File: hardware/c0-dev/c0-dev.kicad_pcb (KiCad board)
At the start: 2 copper layers, 434 parts, among them J101 2913730000, J102 2913710000, J103 2913730000, J104 2913730000, J105 2913710000, J106 2913730000, J107 2913730000, J108 2913710000, J109 2913730000, J110 2913730000, J111 2913730000, J112 2913710000, J113 2913730000, J114 2913730000, J201 RJ45_LED_Shielded, J401 TAG_CONNECT, J402 PinHeader_2.54mm, Q1001 BSS138P, Q1002 BSS138P, Q1003 BSS138P, Q1004 BSS138P, Q1005 BSS138P, Q1006 BSS138P, Q1007 BSS138P, Q1008 BSS138P, Q701 BSS138P, Q702 BSS138P, U1001 B0505S-1WR3, U1002 ISO1540, U1003 TLP175A, U1004 TCA9555PWR, U1005 TPS4H000A-Q1, U1006 TPS4H000A-Q1, U1101 LM5160A, U1102 LM317L, U1201 ER_OLEDM0.91_1x-I2C, U201 LAN8720A, U301 TPS54360DDA, U302 TPS2378, U303 TLP175A, U304 B0505S-1WR3, U305 AMS1117-3.3, U401 TCA9555PWR, U402 W25Q128JVP, U403 TPS3820-33DBV, U404 RP2350A, U501 TMP117xxDRV, U502 B0505S-1WR3, U503 ISO1540, U504 AMS1117-3.3, U505 ADS1015IDGS, U506 ADS1015IDGS, U601 B0505S-1WR3, U602 ISO1540, U603 ADS1015IDGS, U604 ADS1015IDGS, U605 ADS1015IDGS, U606 ADS1015IDGS, U701 B0505S-1WR3, U702 ISO6741, U703 ISO6741, U704 ADS1220xPW, U705 ADS1220xPW, U801 B0505S-1WR3, U802 ISO1044BD, U803 TLP175A, U901 ISO1212, U902 ISO1212, U903 ISO1212, U904 ISO1212, Y401 ABM8-272-T3 (12Mhz)

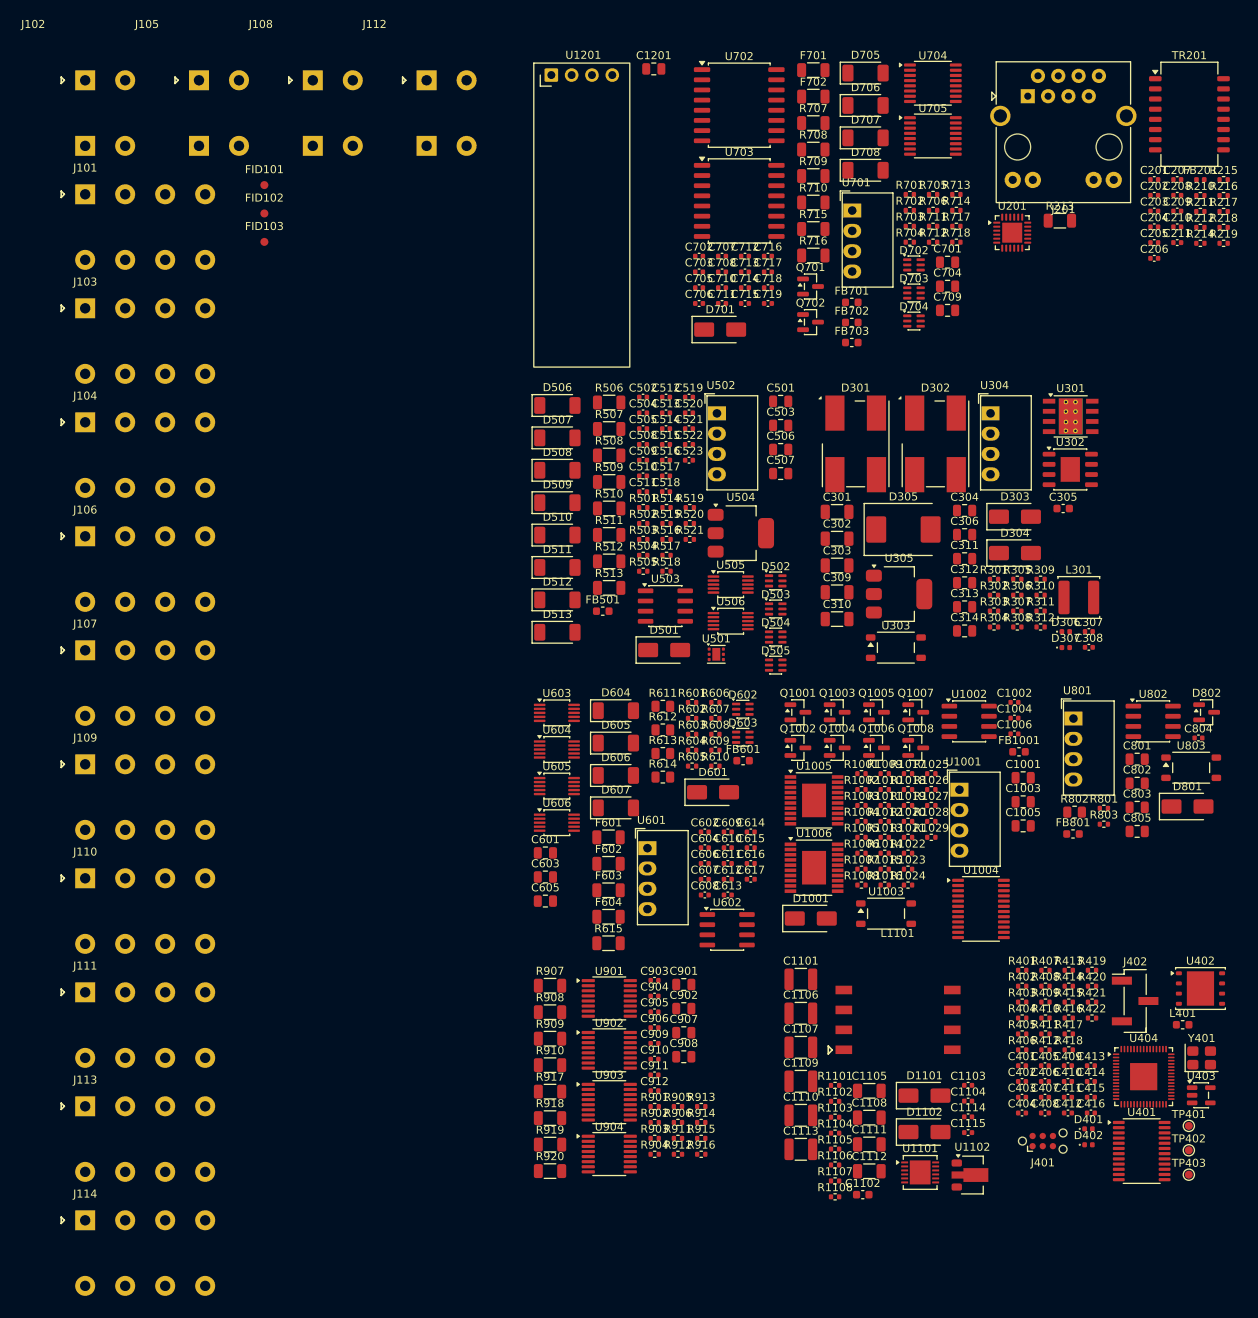
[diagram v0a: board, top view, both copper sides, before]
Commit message: cjc overhaul
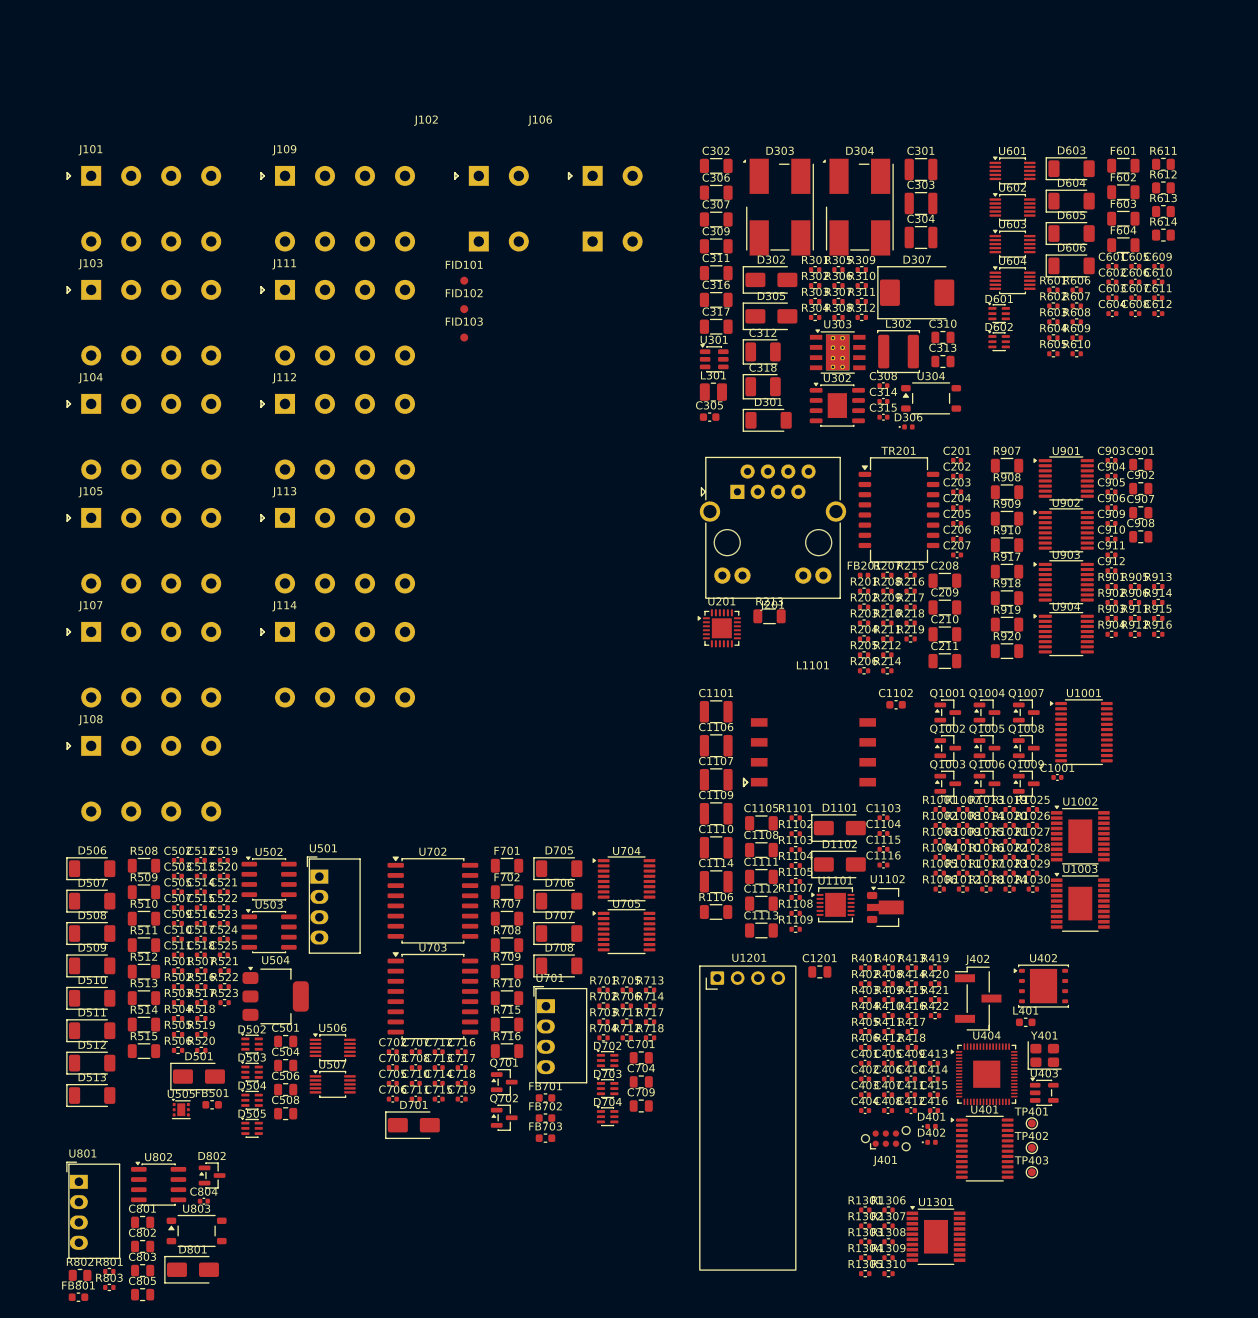
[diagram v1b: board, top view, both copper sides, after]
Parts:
- removed C1002, C1004, C1006, C613, C614, C615, C616, C617: 0.1uF, Capacitor_SMD:C_0402_1005Metric
- removed C1003, C1005: 10uF, Capacitor_SMD:C_0805_2012Metric
- removed D1001: SS14, Diode_SMD:D_SMA
- removed D607: PTVS30VP1UP, Diode_SMD:D_SOD-128
- removed FB1001, FB601: 600Ω@100MHz, Inductor_SMD:L_0603_1608Metric
- removed J110: 2913730000, conduit:2913730000
- removed R615: 0, Resistor_SMD:R_1206_3216Metric
- removed U1004: TCA9555PWR, Package_SO:TSSOP-24_4.4x7.8mm_P0.65mm
- removed U1005, U1006: TPS4H000A-Q1, Package_SO:ETSSOP-20-1EP_4.4x6.5mm_P0.65mm_EP3x4.2mm
- removed U305: AMS1117-3.3, Package_TO_SOT_SMD:SOT-223-3_TabPin2
- removed U605, U606: ADS1015IDGS, Package_SO:TSSOP-10_3x3mm_P0.5mm
- added C1116: 4.7nF, Capacitor_SMD:C_0402_1005Metric, F.Cu at (133.4, 125.0)
- added C315: 3.3nF, Capacitor_SMD:C_0402_1005Metric, F.Cu at (133.4, 69.0)
- added C316: 22uF, Capacitor_SMD:C_1206_3216Metric, F.Cu at (112.5, 54.3)
- added C317: 22uF, Capacitor_SMD:C_1206_3216Metric, F.Cu at (112.5, 57.7)
- added C318: 100uF, Capacitor_Tantalum_SMD:CP_EIA-3528-21_Kemet-B, F.Cu at (118.4, 65.2)
- added C524: 0.1uF, Capacitor_SMD:C_0402_1005Metric, F.Cu at (51.0, 134.2)
- added C525: 0.1uF, Capacitor_SMD:C_0402_1005Metric, F.Cu at (51.0, 136.2)
- added L302: 4.7uH, Inductor_SMD:L_Sunlord_SWPA5040S, F.Cu at (135.3, 60.8)
- added Q1009: BSS138P, Package_TO_SOT_SMD:SOT-23, F.Cu at (151.3, 114.8)
- added R1030: 20k, Resistor_SMD:R_0402_1005Metric, F.Cu at (152.1, 128.0)
- added R1109: 51k, Resistor_SMD:R_0402_1005Metric, F.Cu at (122.5, 133.0)
- added R1301: 1k, Resistor_SMD:R_0402_1005Metric, F.Cu at (131.2, 168.1)
- added R1302: 1k, Resistor_SMD:R_0402_1005Metric, F.Cu at (131.2, 170.1)
- added R1303: 1k, Resistor_SMD:R_0402_1005Metric, F.Cu at (131.2, 172.1)
- added R1304: 1k, Resistor_SMD:R_0402_1005Metric, F.Cu at (131.2, 174.1)
- added R1305: 2.4k, Resistor_SMD:R_0402_1005Metric, F.Cu at (131.2, 176.0)
- added R1306: 1k, Resistor_SMD:R_0402_1005Metric, F.Cu at (134.1, 168.1)
- added R1307: 1k, Resistor_SMD:R_0402_1005Metric, F.Cu at (134.1, 170.1)
- added R1308: 4.7k, Resistor_SMD:R_0402_1005Metric, F.Cu at (134.1, 172.1)
- added R1309: 20k, Resistor_SMD:R_0402_1005Metric, F.Cu at (134.1, 174.1)
- added R1310: 20k, Resistor_SMD:R_0402_1005Metric, F.Cu at (134.1, 176.0)
- added R201: 10k, Resistor_SMD:R_0402_1005Metric, F.Cu at (131.0, 90.7)
- added R202: 1k, Resistor_SMD:R_0402_1005Metric, F.Cu at (131.0, 92.7)
- added R203: 10R, Resistor_SMD:R_0402_1005Metric, F.Cu at (131.0, 94.7)
- added R204: 10R, Resistor_SMD:R_0402_1005Metric, F.Cu at (131.0, 96.7)
- added R205: 10R, Resistor_SMD:R_0402_1005Metric, F.Cu at (131.0, 98.7)
- added R206: 10R, Resistor_SMD:R_0402_1005Metric, F.Cu at (131.0, 100.7)
- added R207: 33R, Resistor_SMD:R_0402_1005Metric, F.Cu at (133.9, 88.7)
- added R208: 12.1k, Resistor_SMD:R_0402_1005Metric, F.Cu at (133.9, 90.7)
- added R209: 49.9R, Resistor_SMD:R_0402_1005Metric, F.Cu at (133.9, 92.7)
- added R522: 1M, Resistor_SMD:R_0402_1005Metric, F.Cu at (51.1, 140.2)
- added R523: 1M, Resistor_SMD:R_0402_1005Metric, F.Cu at (51.1, 142.2)
- added U1301: TPS4H000A-Q1, Package_SO:ETSSOP-20-1EP_4.4x6.5mm_P0.65mm_EP3x4.2mm, F.Cu at (140.0, 171.4)
- added U507: ADS1015IDGS, Package_SO:TSSOP-10_3x3mm_P0.5mm, F.Cu at (64.6, 152.4)
- C1001, C503, C507, C605: value 10uF -> 0.1uF; footprint Capacitor_SMD:C_0805_2012Metric -> Capacitor_SMD:C_0402_1005Metric
- C1113: value 10uF -> 1nF; footprint Capacitor_SMD:C_1210_3225Metric -> Capacitor_SMD:C_1206_3216Metric
- C1114: value 10nF -> 10uF; footprint Capacitor_SMD:C_0402_1005Metric -> Capacitor_SMD:C_1210_3225Metric
- C1115: value 4.7nF -> 10nF
- C208, C209, C210, C211: value 22nF -> 1nF; footprint Capacitor_SMD:C_0402_1005Metric -> Capacitor_SMD:C_1206_3216Metric
- C301, C303: value 1uF -> 10uF; footprint Capacitor_SMD:C_1206_3216Metric -> Capacitor_SMD:C_1210_3225Metric
- C302: value 1uF -> 22uF
- C304: value 0.1uF -> 10uF; footprint Capacitor_SMD:C_0805_2012Metric -> Capacitor_SMD:C_1210_3225Metric
- C306: value 0.1uF -> 1uF; footprint Capacitor_SMD:C_0805_2012Metric -> Capacitor_SMD:C_1206_3216Metric
- C307: value 270pF -> 1uF; footprint Capacitor_SMD:C_0402_1005Metric -> Capacitor_SMD:C_1206_3216Metric
- C308: value 3.3nF -> 0.1uF
- C309: value 22uF -> 1uF
- C310: value 22uF -> 0.1uF; footprint Capacitor_SMD:C_1206_3216Metric -> Capacitor_SMD:C_0805_2012Metric
- C311: value 10uF -> 22uF; footprint Capacitor_SMD:C_0805_2012Metric -> Capacitor_SMD:C_1206_3216Metric
- C312: value 10uF -> 100uF; footprint Capacitor_SMD:C_0805_2012Metric -> Capacitor_Tantalum_SMD:CP_EIA-3528-21_Kemet-B
- C313: value 10uF -> 0.1uF
- C314: value 10uF -> 270pF; footprint Capacitor_SMD:C_0805_2012Metric -> Capacitor_SMD:C_0402_1005Metric
- C504: value 0.1uF -> 10uF; footprint Capacitor_SMD:C_0402_1005Metric -> Capacitor_SMD:C_0805_2012Metric
- C508: value 1uF -> 10uF; footprint Capacitor_SMD:C_0402_1005Metric -> Capacitor_SMD:C_0805_2012Metric
- C510, C602, C604: value 0.1uF -> 1uF
- C601, C603: value 10uF -> 1uF; footprint Capacitor_SMD:C_0805_2012Metric -> Capacitor_SMD:C_0402_1005Metric
- C606, C607, C608, C609: value 1uF -> 0.1uF
- D301: value CD-DF406SL -> PTVS30VP1UP; footprint Diode_SMD:Diode_Bridge_Bourns_CD-DF4xxS -> Diode_SMD:D_SOD-128
- D302: value CD-DF406SL -> SS14; footprint Diode_SMD:Diode_Bridge_Bourns_CD-DF4xxS -> Diode_SMD:D_SMA
- D303: value SMAJ58A -> CD-DF406SL; footprint Diode_SMD:D_SMA -> Diode_SMD:Diode_Bridge_Bourns_CD-DF4xxS
- D304: value SS14 -> CD-DF406SL; footprint Diode_SMD:D_SMA -> Diode_SMD:Diode_Bridge_Bourns_CD-DF4xxS
- D305: value B560C -> SMAJ58A; footprint Diode_SMD:D_SMC -> Diode_SMD:D_SMA
- D307: value green -> B560C; footprint LED_SMD:LED_0402_1005Metric -> Diode_SMD:D_SMC
- D601: value SS14 -> BAV199DW; footprint Diode_SMD:D_SMA -> Package_TO_SOT_SMD:SOT-363_SC-70-6
- D603: value BAV199DW -> PTVS30VP1UP; footprint Package_TO_SOT_SMD:SOT-363_SC-70-6 -> Diode_SMD:D_SOD-128
- J105, J108, J112: value 2913710000 -> 2913730000; footprint conduit:2913710000 -> conduit:2913730000
- J106: value 2913730000 -> 2913710000; footprint conduit:2913730000 -> conduit:2913710000
- L301: value 4.7uH -> 2.2uH; footprint Inductor_SMD:L_Sunlord_SWPA5040S -> Inductor_SMD:L_1008_2520Metric
- R1001, R1002, R1009, R1012: value 1k -> 4.7k
- R1007: value 10k -> 1k
- R1008: value 4.7k -> 10k
- R1011: value 4.7k -> 1k
- R1022: value 20k -> 1k
- R1106: value 27k -> 2M; footprint Resistor_SMD:R_0402_1005Metric -> Resistor_SMD:R_1206_3216Metric
- R1107: value 2.4k -> 27k
- R1108: value 51k -> 2.4k
- R301: value 68.1k -> 1k
- R302: value 0 -> 25k
- R303: value 25k -> 63.4R
- R304: value 63.4R -> 68.1k
- R305: value 6.34k -> 1k
- R306: value 60.4k -> 1k
- R307: value 11.5k -> 10k
- R309: value 10k -> 6.34k
- R310: value 1k -> 60.4k
- R311: value 1k -> 11.5k
- R506, R507: value 2k -> 1k; footprint Resistor_SMD:R_1206_3216Metric -> Resistor_SMD:R_0402_1005Metric
- R514, R515: value 1M -> 2k; footprint Resistor_SMD:R_0402_1005Metric -> Resistor_SMD:R_1206_3216Metric
- R611, R612, R613, R614: value 160 -> 82
- U1001: value B0505S-1WR3 -> TCA9555PWR; footprint Converter_DCDC:Converter_DCDC_Murata_MEE1SxxxxSC_THT -> Package_SO:TSSOP-24_4.4x7.8mm_P0.65mm
- U1002: value ISO1540 -> TPS4H000A-Q1; footprint Package_SO:SOIC-8_3.9x4.9mm_P1.27mm -> Package_SO:ETSSOP-20-1EP_4.4x6.5mm_P0.65mm_EP3x4.2mm
- U1003: value TLP175A -> TPS4H000A-Q1; footprint Package_SO:Toshiba_SOIC-4-6_4.4x3.6mm_P1.27mm -> Package_SO:ETSSOP-20-1EP_4.4x6.5mm_P0.65mm_EP3x4.2mm
- U301: value TPS54360DDA -> AP63203WU; footprint Package_SO:TI_SO-PowerPAD-8_ThermalVias -> Package_TO_SOT_SMD:TSOT-23-6
- U303: value TLP175A -> TPS54360DDA; footprint Package_SO:Toshiba_SOIC-4-6_4.4x3.6mm_P1.27mm -> Package_SO:TI_SO-PowerPAD-8_ThermalVias
- U304: value B0505S-1WR3 -> TLP175A; footprint Converter_DCDC:Converter_DCDC_Murata_MEE1SxxxxSC_THT -> Package_SO:Toshiba_SOIC-4-6_4.4x3.6mm_P1.27mm
- U501: value TMP117xxDRV -> B0505S-1WR3; footprint Package_SON:WSON-6-1EP_2x2mm_P0.65mm_EP1x1.6mm -> Converter_DCDC:Converter_DCDC_Murata_MEE1SxxxxSC_THT
- U502: value B0505S-1WR3 -> ISO1540; footprint Converter_DCDC:Converter_DCDC_Murata_MEE1SxxxxSC_THT -> Package_SO:SOIC-8_3.9x4.9mm_P1.27mm
- U505: value ADS1015IDGS -> TMP117xxDRV; footprint Package_SO:TSSOP-10_3x3mm_P0.5mm -> Package_SON:WSON-6-1EP_2x2mm_P0.65mm_EP1x1.6mm
- U601: value B0505S-1WR3 -> ADS1015IDGS; footprint Converter_DCDC:Converter_DCDC_Murata_MEE1SxxxxSC_THT -> Package_SO:TSSOP-10_3x3mm_P0.5mm
- U602: value ISO1540 -> ADS1015IDGS; footprint Package_SO:SOIC-8_3.9x4.9mm_P1.27mm -> Package_SO:TSSOP-10_3x3mm_P0.5mm
- moved C802 137.1 mm to (40.8, 172.6)
- moved C804 137.1 mm to (48.5, 167.0)
- moved D801 137.1 mm to (47.1, 175.6)
- moved D802 137.1 mm to (49.5, 163.8)
- moved FB801 137.1 mm to (32.8, 179.0)
- moved R801 137.1 mm to (36.7, 175.8)
- moved R802 137.1 mm to (33.0, 176.3)
- moved U803 137.1 mm to (47.6, 170.7)
- moved C801 137.1 mm to (40.8, 169.6)
- moved C803 137.1 mm to (40.8, 175.7)
- moved C805 137.1 mm to (40.8, 178.7)
- moved R803 137.1 mm to (36.7, 177.8)
- moved U801 137.1 mm to (32.9, 164.6)
- moved U802 137.1 mm to (42.8, 164.9)
- moved U1201 114.8 mm to (112.7, 139.1)
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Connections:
- net /frontend_temp/+5V renamed /frontend_temp/+5V_ISO
- C1001 pad 1: +5V_ISO -> +3.3V
- C1001 pad 2: GND_ISO -> GND
- C1101 pad 2: GND_ISO -> /Power/GND_ISO
- C1102 pad 2: GND_ISO -> /Power/GND_ISO
- C1103 pad 2: GND_ISO -> /Power/GND_ISO
- C1105 pad 2: GND_ISO -> /Power/GND_ISO
- C1106 pad 1: /Power/FlyBuck/+24V -> +24V
- C1106 pad 2: /Power/FlyBuck/GND -> GND
- C1107 pad 1: /Power/FlyBuck/+24V -> +24V
- C1107 pad 2: /Power/FlyBuck/GND -> GND
- C1108 pad 1: /Power/FlyBuck/+24V -> +24V
- C1108 pad 2: /Power/FlyBuck/GND -> GND
- C1109 pad 1: /Power/FlyBuck/+24V -> +24V
- C1109 pad 2: /Power/FlyBuck/GND -> GND
- C1110 pad 1: /Power/FlyBuck/+24V -> +24V
- C1110 pad 2: /Power/FlyBuck/GND -> GND
- C1111 pad 1: /Power/FlyBuck/+24V -> +24V
- C1111 pad 2: /Power/FlyBuck/GND -> GND
- C1112 pad 1: /Power/FlyBuck/+24V -> +24V
- C1112 pad 2: GND_ISO -> /Power/GND_ISO
- C1113 pad 1: /Power/FlyBuck/+24V -> GND
- C1113 pad 2: GND_ISO -> Earth
- C1114 pad 1: /Power/FlyBuck/A -> +24V
- C1114 pad 2: /Power/FlyBuck/FB -> /Power/GND_ISO
- C1115 pad 2: GND_ISO -> /Power/FlyBuck/FB
- C301 pad 1: +POE -> +24V
- C301 pad 2: GND_ISO -> GND
- C302 pad 1: +POE -> +5V
- C302 pad 2: GND_ISO -> GND
- C303 pad 1: +POE -> +24V
- C303 pad 2: GND_ISO -> GND
- C304 pad 1: +POE -> +24V
- C304 pad 2: GND_ISO -> GND
- C306 pad 1: Net-(U301-BOOT) -> +24V
- C306 pad 2: Net-(D305-K) -> GND
- C307 pad 1: Net-(U301-COMP) -> +24V
- C307 pad 2: GND_ISO -> GND
- C308 pad 1: Net-(C308-Pad1) -> Net-(U301-SW)
- C308 pad 2: GND_ISO -> Net-(U301-BST)
- C309 pad 1: +5V_ISO -> +24V
- C309 pad 2: GND_ISO -> GND
- C310 pad 1: +5V_ISO -> +24V
- C310 pad 2: GND_ISO -> GND
- C311 pad 1: +5V_ISO -> GND
- C311 pad 2: GND_ISO -> +3.3V
- C312 pad 1: +5V -> +3.3V
- C313 pad 1: +5V -> Net-(U303-BOOT)
- C313 pad 2: GND -> Net-(D307-K)
- C314 pad 1: +3.3V -> Net-(U303-COMP)
- C501 pad 1: +5V_ISO -> +5V
- C501 pad 2: GND_ISO -> GND
- C503 pad 1: unconnected-(C503-Pad1) -> +3.3V
- C504 pad 1: +3.3V -> unconnected-(C504-Pad1)
- C512 pad 1: Net-(D502B-K1A2) -> +3.3V
- C513 pad 1: Net-(D502B-K1A2) -> +3.3V
- C513 pad 2: Net-(D502A-K3A4) -> GND
- C514 pad 1: Net-(D502A-K3A4) -> Net-(D502B-K1A2)
- C515 pad 1: Net-(D503B-K1A2) -> Net-(D502B-K1A2)
- C515 pad 2: GND -> Net-(D502A-K3A4)
- C516 pad 1: Net-(D503B-K1A2) -> Net-(D502A-K3A4)
- C516 pad 2: Net-(D503A-K3A4) -> GND
- C517 pad 1: Net-(D503A-K3A4) -> Net-(D503B-K1A2)
- C518 pad 1: Net-(D504B-K1A2) -> Net-(D503B-K1A2)
- C518 pad 2: GND -> Net-(D503A-K3A4)
- C519 pad 1: Net-(D504B-K1A2) -> Net-(D503A-K3A4)
- C519 pad 2: Net-(D504A-K3A4) -> GND
- C520 pad 1: Net-(D504A-K3A4) -> Net-(D504B-K1A2)
- C521 pad 1: Net-(D505B-K1A2) -> Net-(D504B-K1A2)
- C521 pad 2: GND -> Net-(D504A-K3A4)
- C522 pad 1: Net-(D505B-K1A2) -> Net-(D504A-K3A4)
- C522 pad 2: Net-(D505A-K3A4) -> GND
- C523 pad 1: Net-(D505A-K3A4) -> Net-(D505B-K1A2)
- C601 pad 1: +5V_ISO -> +3.3V
- C601 pad 2: GND_ISO -> GND
- C603 pad 1: Net-(U601-+Vout) -> +3.3V
- C604 pad 1: /frontend_420/+5V -> +3.3V
- C605 pad 1: /frontend_420/+5V -> +3.3V
- C606 pad 1: /frontend_420/+5V -> +3.3V
- C607 pad 1: /frontend_420/+5V -> +3.3V
- C608 pad 1: /frontend_420/+5V -> +3.3V
- C609 pad 1: /frontend_420/+5V -> GND
- C609 pad 2: GND -> Net-(U601-AIN0)
- C610 pad 1: /frontend_420/+5V -> GND
- C610 pad 2: GND -> Net-(U602-AIN0)
- C611 pad 1: /frontend_420/+5V -> GND
- C611 pad 2: GND -> Net-(U603-AIN0)
- C612 pad 1: /frontend_420/+5V -> GND
- C612 pad 2: GND -> Net-(U604-AIN0)
- C903 pad 2: /Digital Input/GND_IN -> GND
- C904 pad 2: /Digital Input/GND_IN -> GND
- C905 pad 2: /Digital Input/GND_IN -> GND
- C906 pad 2: /Digital Input/GND_IN -> GND
- C909 pad 2: /Digital Input/GND_IN -> GND
- C910 pad 2: /Digital Input/GND_IN -> GND
- C911 pad 2: /Digital Input/GND_IN -> GND
- C912 pad 2: /Digital Input/GND_IN -> GND
- D1101 pad 1: /Power/FlyBuck/+24V -> +24V
- D1102 pad 1: /Power/FlyBuck/+24V -> +24V
- D301 pad 1: +POE -> GND
- D301 pad 2: /Ethernet/POE+12 -> /Power/V+
- D302 pad 1: +POE -> +24V
- D302 pad 2: /Ethernet/POE+45 -> /Power/V+
- D303 pad 2: -POE -> /Ethernet/POE+12
- D304 pad 2: /Power/V+ -> /Ethernet/POE+45
- D305 pad 1: Net-(D305-K) -> +POE
- D305 pad 2: GND_ISO -> -POE
- D306 pad 1: GND_ISO -> GND
- D307 pad 1: GND -> Net-(D307-K)
- D307 pad 2: Net-(D307-A) -> GND
- D601 pad 1: /frontend_420/+5V -> GND
- D601 pad 2: Net-(D601-A) -> +3.3V
- D602 pad 2: /frontend_420/+5V -> +3.3V
- D602 pad 5: /frontend_420/+5V -> +3.3V
- D603 pad 1: GND -> /frontend_420/4200
- D603 pad 2: /frontend_420/+5V -> GND
- D604 pad 1: /frontend_420/4200 -> /frontend_420/4201
- D605 pad 1: /frontend_420/4201 -> /frontend_420/4202
- D606 pad 1: /frontend_420/4202 -> /frontend_420/4203
- F601 pad 1: Net-(D602A-K3A4) -> Net-(D601A-K3A4)
- F602 pad 1: Net-(D602B-K1A2) -> Net-(D601B-K1A2)
- F603 pad 1: Net-(D603A-K3A4) -> Net-(D602A-K3A4)
- F604 pad 1: Net-(D603B-K1A2) -> Net-(D602B-K1A2)
- FB501 pad 1: Net-(U502-+Vout) -> Net-(U501-+Vout)
- J103 pad 1: /Digital Input/IN0 -> /Power Output/OUT0
- J103 pad 2: /Digital Input/IN1 -> /Power Output/OUT1
- J103 pad 3: /Digital Input/IN2 -> GND
- J103 pad 4: /Digital Input/IN3 -> GND
- J104 pad 1: /Digital Input/IN4 -> /Digital Input/IN0
- J104 pad 2: /Digital Input/IN5 -> /Digital Input/IN1
- J104 pad 3: /Digital Input/IN6 -> /Digital Input/IN2
- J104 pad 4: /Digital Input/IN7 -> /Digital Input/IN3
- J105 pad 1: /Digital Input/GND_IN -> /Digital Input/IN4
- J105 pad 2: /Digital Input/GND_IN -> /Digital Input/IN5
- J106 pad 1: /frontend_temp/TC0+ -> GND
- J106 pad 2: /frontend_temp/TC0- -> GND
- J107 pad 1: /frontend_temp/TC2+ -> /Digital Output/OUT0
- J107 pad 2: /frontend_temp/TC2- -> /Digital Output/OUT1
- J107 pad 3: /frontend_temp/TC3+ -> /Digital Output/OUT2
- J107 pad 4: /frontend_temp/TC3- -> /Digital Output/OUT3
- J108 pad 1: VS -> /Digital Output/OUT4
- J108 pad 2: GND -> /Digital Output/OUT5
- J109 pad 1: /Digital Output/OUT0 -> /frontend_420/4200
- J109 pad 2: /Digital Output/OUT1 -> /frontend_420/4201
- J109 pad 3: /Digital Output/OUT2 -> /frontend_420/4202
- J109 pad 4: /Digital Output/OUT3 -> /frontend_420/4203
- J111 pad 1: /frontend_420/4200 -> /frontend_temp/TC0+
- J111 pad 2: /frontend_420/4201 -> /frontend_temp/TC0-
- J111 pad 3: /frontend_420/4202 -> /frontend_temp/TC1+
- J111 pad 4: /frontend_420/4203 -> /frontend_temp/TC1-
- J112 pad 1: /frontend_420/420_GND -> /frontend_temp/TC2+
- J112 pad 2: /frontend_420/420_GND -> /frontend_temp/TC2-
- L1101 pad 2: (no net) -> unconnected-(L1101-Pad2)
- L1101 pad 4: /Power/FlyBuck/GND -> GND
- L1101 pad 6: /Power/FlyBuck/GND -> GND
- L1101 pad 7: (no net) -> unconnected-(L1101-Pad7)
- L1101 pad 8: /Power/FlyBuck/+24V -> +24V
- L301 pad 1: Net-(D305-K) -> Net-(U301-SW)
- L301 pad 2: +5V_ISO -> +3.3V
- Q1001 pad 1: /Digital Output/~{EN} -> /EN
- Q1001 pad 3: /Digital Output/P00 -> /Digital Output/~{EN}
- Q1002 pad 3: /Digital Output/P06 -> /Digital Output/P00
- Q1003 pad 3: /Digital Output/P01 -> /Digital Output/P04
- Q1004 pad 3: /Digital Output/P07 -> /Digital Output/P01
- Q1005 pad 3: /Digital Output/P02 -> /Digital Output/P05
- Q1006 pad 3: /Digital Output/P03 -> /Digital Output/P02
- Q1007 pad 3: /Digital Output/P04 -> /Digital Output/P06
- Q1008 pad 3: /Digital Output/P05 -> /Digital Output/P03
- R1001 pad 1: /Digital Output/~{EN} -> GND
- R1001 pad 2: +3.3V -> /EN
- R1002 pad 1: GND -> /Digital Output/~{EN}
- R1002 pad 2: Net-(U1004-A1) -> +3.3V
- R1003 pad 2: /Digital Output/+5V -> +3.3V
- R1004 pad 2: /Digital Output/+5V -> +3.3V
- R1005 pad 2: Net-(U1004-A2) -> Net-(U1001-A2)
- R1006 pad 2: Net-(U1004-A0) -> Net-(U1001-A1)
- R1007 pad 1: Net-(U1004-~{INT}) -> GND
- R1007 pad 2: /Digital Output/+5V -> Net-(U1001-A0)
- R1008 pad 1: GND -> Net-(U1001-~{INT})
- R1008 pad 2: Net-(U1005-CL) -> +3.3V
- R1009 pad 1: /Digital Output/+5V -> GND
- R1009 pad 2: Net-(U1005-DIAG_EN) -> Net-(U1002-CL)
- R1010 pad 1: GND -> +3.3V
- R1010 pad 2: Net-(U1005-THER) -> Net-(U1002-DIAG_EN)
- R1011 pad 2: Net-(U1006-CL) -> Net-(U1002-THER)
- R1012 pad 1: /Digital Output/+5V -> GND
- R1012 pad 2: Net-(U1006-DIAG_EN) -> Net-(U1003-CL)
- R1013 pad 1: GND -> +3.3V
- R1013 pad 2: Net-(U1006-THER) -> Net-(U1003-DIAG_EN)
- R1014 pad 1: /Digital Output/~{FLT0} -> GND
- R1014 pad 2: /Digital Output/+5V -> Net-(U1003-THER)
- R1015 pad 1: /Digital Output/~{FLT1} -> /Digital Output/~{FLT0}
- R1015 pad 2: /Digital Output/+5V -> +3.3V
- R1016 pad 1: /Digital Output/~{FLT2} -> /Digital Output/~{FLT1}
- R1016 pad 2: /Digital Output/+5V -> +3.3V
- R1017 pad 1: /Digital Output/~{FLT3} -> /Digital Output/~{FLT2}
- R1017 pad 2: /Digital Output/+5V -> +3.3V
- R1018 pad 1: /Digital Output/~{FLT4} -> /Digital Output/~{FLT3}
- R1018 pad 2: /Digital Output/+5V -> +3.3V
- R1019 pad 1: /Digital Output/~{FLT5} -> /Digital Output/~{FLT4}
- R1019 pad 2: /Digital Output/+5V -> +3.3V
- R1020 pad 1: /Digital Output/~{FLT6} -> /Digital Output/~{FLT5}
- R1020 pad 2: /Digital Output/+5V -> +3.3V
- R1021 pad 1: /Digital Output/~{FLT7} -> /Digital Output/~{FLT6}
- R1021 pad 2: /Digital Output/+5V -> +3.3V
- R1022 pad 1: /Digital Output/OUT0 -> /Digital Output/~{FLT7}
- R1022 pad 2: VS -> +3.3V
- R1023 pad 1: /Digital Output/OUT1 -> /Digital Output/OUT0
- R1023 pad 2: VS -> +24V
- R1024 pad 1: /Digital Output/OUT2 -> /Digital Output/OUT1
- R1024 pad 2: VS -> +24V
- R1025 pad 1: /Digital Output/OUT3 -> /Digital Output/OUT2
- R1025 pad 2: VS -> +24V
- R1026 pad 1: /Digital Output/OUT4 -> /Digital Output/OUT3
- R1026 pad 2: VS -> +24V
- R1027 pad 1: /Digital Output/OUT5 -> /Digital Output/OUT4
- R1027 pad 2: VS -> +24V
- R1028 pad 1: /Digital Output/OUT6 -> /Digital Output/OUT5
- R1028 pad 2: VS -> +24V
- R1029 pad 1: /Digital Output/OUT7 -> /Digital Output/OUT6
- R1029 pad 2: VS -> +24V
- R1105 pad 2: GND_ISO -> /Power/GND_ISO
- R1106 pad 1: /Power/FlyBuck/+24V -> Earth
- R1106 pad 2: /Power/FlyBuck/FB -> GND
- R1107 pad 1: /Power/FlyBuck/FB -> +24V
- R1107 pad 2: GND_ISO -> /Power/FlyBuck/FB
- R1108 pad 1: /Power/FlyBuck/SW -> /Power/FlyBuck/FB
- R1108 pad 2: /Power/FlyBuck/A -> /Power/GND_ISO
- R301 pad 1: Net-(U301-RT/CLK) -> Net-(U301-EN)
- R301 pad 2: GND_ISO -> +5V
- R302 pad 1: GND_ISO -> Net-(U302-DEN)
- R302 pad 2: GND -> +POE
- R303 pad 1: Net-(U302-DEN) -> -POE
- R303 pad 2: +POE -> Net-(U302-CLS)
- R304 pad 1: -POE -> Net-(U303-RT/CLK)
- R304 pad 2: Net-(U302-CLS) -> GND
- R305 pad 1: Net-(U301-COMP) -> Net-(U303-EN)
- R305 pad 2: Net-(C308-Pad1) -> +24V
- R306 pad 1: +5V_ISO -> /Power/GND_ISO
- R306 pad 2: Net-(R306-Pad2) -> Net-(U302-APD)
- R307 pad 1: Net-(R306-Pad2) -> +POE
- R307 pad 2: GND_ISO -> Net-(R307-Pad2)
- R308 pad 1: GND_ISO -> Net-(D306-A)
- R308 pad 2: Net-(U302-APD) -> +3.3V
- R309 pad 1: +POE -> Net-(U303-COMP)
- R309 pad 2: Net-(R309-Pad2) -> Net-(C315-Pad1)
- R310 pad 1: Net-(D306-A) -> +5V
- R310 pad 2: +5V_ISO -> /Power/FB2
- R311 pad 1: +3.3V -> /Power/FB2
- R311 pad 2: /MCU/POE_T2P -> GND
- R312 pad 1: Net-(D307-A) -> +3.3V
- R312 pad 2: +3.3V -> /MCU/POE_T2P
- R406 pad 2: Net-(U401-P04) -> Net-(U401-P05)
- R407 pad 2: Net-(U401-P05) -> Net-(U401-P06)
- R501 pad 1: GND -> /MCU/I2C0.SCL
- R501 pad 2: Net-(U501-ADD0) -> +3.3V
- R502 pad 1: /MCU/I2C0.SCL -> /frontend_temp/SDA_400k
- R504 pad 1: GND -> /frontend_temp/SCL_400k
- R504 pad 2: Net-(U505-ADDR) -> +3.3V
- R505 pad 1: +3.3V -> GND
- R506 pad 1: /frontend_temp/TC0- -> GND
- R506 pad 2: Net-(D502B-K1A2) -> Net-(U505-ADD0)
- R507 pad 1: /frontend_temp/TC0+ -> +3.3V
- R507 pad 2: Net-(D502A-K3A4) -> Net-(U507-ADDR)
- R508 pad 1: /frontend_temp/TC1- -> /frontend_temp/TC0-
- R508 pad 2: Net-(D503B-K1A2) -> Net-(D502B-K1A2)
- R509 pad 1: /frontend_temp/TC1+ -> /frontend_temp/TC0+
- R509 pad 2: Net-(D503A-K3A4) -> Net-(D502A-K3A4)
- R510 pad 1: /frontend_temp/TC2- -> /frontend_temp/TC1-
- R510 pad 2: Net-(D504B-K1A2) -> Net-(D503B-K1A2)
- R511 pad 1: /frontend_temp/TC2+ -> /frontend_temp/TC1+
- R511 pad 2: Net-(D504A-K3A4) -> Net-(D503A-K3A4)
- R512 pad 1: /frontend_temp/TC3- -> /frontend_temp/TC2-
- R512 pad 2: Net-(D505B-K1A2) -> Net-(D504B-K1A2)
- R513 pad 1: /frontend_temp/TC3+ -> /frontend_temp/TC2+
- R513 pad 2: Net-(D505A-K3A4) -> Net-(D504A-K3A4)
- R514 pad 1: /frontend_temp/TC0- -> /frontend_temp/TC3-
- R514 pad 2: +3.3V -> Net-(D505B-K1A2)
- R515 pad 1: GND -> /frontend_temp/TC3+
- R515 pad 2: /frontend_temp/TC0+ -> Net-(D505A-K3A4)
- R516 pad 1: /frontend_temp/TC1- -> /frontend_temp/TC0-
- R517 pad 2: /frontend_temp/TC1+ -> /frontend_temp/TC0+
- R518 pad 1: /frontend_temp/TC2- -> /frontend_temp/TC1-
- R519 pad 2: /frontend_temp/TC2+ -> /frontend_temp/TC1+
- R520 pad 1: /frontend_temp/TC3- -> /frontend_temp/TC2-
- R521 pad 2: /frontend_temp/TC3+ -> /frontend_temp/TC2+
- R601 pad 1: /MCU/I2C2.SCL -> /I2C2.SCL
- R601 pad 2: /frontend_420/+5V -> +3.3V
- R602 pad 1: /MCU/I2C2.SDA -> /I2C2.SDA
- R602 pad 2: /frontend_420/+5V -> +3.3V
- R603 pad 2: Net-(U603-ADDR) -> Net-(U601-ADDR)
- R604 pad 2: Net-(U604-ADDR) -> Net-(U602-ADDR)
- R605 pad 1: /MCU/I2C2.SDA -> /I2C2.SDA
- R605 pad 2: Net-(U605-ADDR) -> Net-(U603-ADDR)
- R606 pad 1: /MCU/I2C2.SCL -> /I2C2.SCL
- R606 pad 2: Net-(U606-ADDR) -> Net-(U604-ADDR)
- R607 pad 1: Net-(U603-AIN0) -> Net-(U601-AIN0)
- R607 pad 2: Net-(D602A-K3A4) -> Net-(D601A-K3A4)
- R608 pad 1: Net-(U604-AIN0) -> Net-(U602-AIN0)
- R608 pad 2: Net-(D602B-K1A2) -> Net-(D601B-K1A2)
- R609 pad 1: Net-(U605-AIN0) -> Net-(U603-AIN0)
- R609 pad 2: Net-(D603A-K3A4) -> Net-(D602A-K3A4)
- R610 pad 1: Net-(U606-AIN0) -> Net-(U604-AIN0)
- R610 pad 2: Net-(D603B-K1A2) -> Net-(D602B-K1A2)
- R611 pad 1: Net-(D602A-K3A4) -> Net-(D601A-K3A4)
- R612 pad 1: Net-(D602B-K1A2) -> Net-(D601B-K1A2)
- R613 pad 1: Net-(D603A-K3A4) -> Net-(D602A-K3A4)
- R614 pad 1: Net-(D603B-K1A2) -> Net-(D602B-K1A2)
- U1001 pad 1: GND_ISO -> Net-(U1001-~{INT})
- U1001 pad 2: +5V_ISO -> Net-(U1001-A1)
- U1001 pad 3: GND -> Net-(U1001-A2)
- U1001 pad 4: Net-(U1001-+Vout) -> /Digital Output/P00
- U1002 pad 1: +3.3V -> /Digital Output/P00
- U1002 pad 2: /MCU/I2C1.SCL -> /Digital Output/P01
- U1002 pad 3: /MCU/I2C1.SDA -> /Digital Output/P02
- U1002 pad 4: GND -> /Digital Output/P03
- U1002 pad 5: GND -> /Digital Output/~{FLT0}
- U1002 pad 6: /MCU/I2C1.SDA -> /Digital Output/~{FLT1}
- U1002 pad 7: /MCU/I2C1.SCL -> /Digital Output/~{FLT2}
- U1002 pad 8: /Digital Output/+5V -> /Digital Output/~{FLT3}
- U1003 pad 1: /EN -> /Digital Output/P04
- U1003 pad 3: GND -> /Digital Output/P06
- U1003 pad 4: GND -> /Digital Output/P07
- U1003 pad 6: /Digital Output/~{EN} -> /Digital Output/~{FLT5}
- U1101 pad 1: GND_ISO -> /Power/GND_ISO
- U1101 pad 13: GND_ISO -> /Power/GND_ISO
- U1101 pad 2: GND_ISO -> /Power/GND_ISO
- U1102 pad 3: /Power/FlyBuck/+24V -> +24V
- U301 pad 1: Net-(U301-BOOT) -> +3.3V
- U301 pad 2: +POE -> Net-(U301-EN)
- U301 pad 3: +POE -> +5V
- U301 pad 4: Net-(U301-RT/CLK) -> GND
- U301 pad 5: /Power/FB -> Net-(U301-SW)
- U301 pad 6: Net-(U301-COMP) -> Net-(U301-BST)
- U302 pad 5: GND_ISO -> /Power/GND_ISO
- U303 pad 1: Net-(R309-Pad2) -> Net-(U303-BOOT)
- U303 pad 3: Net-(U302-T2P) -> Net-(U303-EN)
- U303 pad 4: GND -> Net-(U303-RT/CLK)
- U303 pad 6: /MCU/POE_T2P -> Net-(U303-COMP)
- U304 pad 1: GND_ISO -> Net-(R307-Pad2)
- U304 pad 3: GND -> Net-(U302-T2P)
- U304 pad 4: +5V -> GND
- U401 pad 10: unconnected-(U401-P06-Pad10) -> Net-(U401-P06)
- U401 pad 8: Net-(U401-P04) -> /FAULT_420
- U501 pad 1: /MCU/I2C1.SCL -> GND
- U501 pad 2: GND -> +5V
- U501 pad 3: unconnected-(U501-ALERT-Pad3) -> GND
- U501 pad 4: Net-(U501-ADD0) -> Net-(U501-+Vout)
- U502 pad 1: GND_ISO -> +3.3V
- U502 pad 2: +5V_ISO -> /MCU/I2C0.SDA
- U502 pad 3: GND -> /MCU/I2C0.SCL
- U502 pad 4: Net-(U502-+Vout) -> GND
- U503 pad 2: /MCU/I2C0.SDA -> /MCU/I2C1.SDA
- U503 pad 3: /MCU/I2C0.SCL -> /MCU/I2C1.SCL
- U503 pad 6: /MCU/I2C0.SCL -> /frontend_temp/SCL_400k
- U503 pad 7: /MCU/I2C0.SDA -> /frontend_temp/SDA_400k
- U505 pad 1: Net-(U505-ADDR) -> /frontend_temp/SCL_400k
- U505 pad 2: unconnected-(U505-ALERT/RDY-Pad2) -> GND
- U505 pad 3: GND -> unconnected-(U505-ALERT-Pad3)
- U505 pad 4: Net-(D502B-K1A2) -> Net-(U505-ADD0)
- U505 pad 5: Net-(D502A-K3A4) -> +3.3V
- U505 pad 6: Net-(D503B-K1A2) -> /frontend_temp/SDA_400k
- U505 pad 7: Net-(D503A-K3A4) -> (no net)
- U506 pad 4: Net-(D504B-K1A2) -> Net-(D502B-K1A2)
- U506 pad 5: Net-(D504A-K3A4) -> Net-(D502A-K3A4)
- U506 pad 6: Net-(D505B-K1A2) -> Net-(D503B-K1A2)
- U506 pad 7: Net-(D505A-K3A4) -> Net-(D503A-K3A4)
- U601 pad 1: GND_ISO -> Net-(U601-ADDR)
- U601 pad 2: +5V_ISO -> unconnected-(U601-ALERT/RDY-Pad2)
- U601 pad 4: Net-(U601-+Vout) -> Net-(U601-AIN0)
- U602 pad 1: +3.3V -> Net-(U602-ADDR)
- U602 pad 2: /MCU/I2C2.SDA -> unconnected-(U602-ALERT/RDY-Pad2)
- U602 pad 3: /MCU/I2C2.SCL -> GND
- U602 pad 4: GND -> Net-(U602-AIN0)
- U602 pad 5: GND -> unconnected-(U602-AIN1-Pad5)
- U602 pad 6: /MCU/I2C2.SCL -> unconnected-(U602-AIN2-Pad6)
- U602 pad 7: /MCU/I2C2.SDA -> unconnected-(U602-AIN3-Pad7)
- U602 pad 8: /frontend_420/+5V -> +3.3V
- U603 pad 10: /MCU/I2C2.SCL -> /I2C2.SCL
- U603 pad 8: /frontend_420/+5V -> +3.3V
- U603 pad 9: /MCU/I2C2.SDA -> /I2C2.SDA
- U604 pad 10: /MCU/I2C2.SCL -> /I2C2.SCL
- U604 pad 8: /frontend_420/+5V -> +3.3V
- U604 pad 9: /MCU/I2C2.SDA -> /I2C2.SDA
- U901 pad 14: /Digital Input/GND_IN -> GND
- U901 pad 9: /Digital Input/GND_IN -> GND
- U902 pad 14: /Digital Input/GND_IN -> GND
- U902 pad 9: /Digital Input/GND_IN -> GND
- U903 pad 14: /Digital Input/GND_IN -> GND
- U903 pad 9: /Digital Input/GND_IN -> GND
- U904 pad 14: /Digital Input/GND_IN -> GND
- U904 pad 9: /Digital Input/GND_IN -> GND
